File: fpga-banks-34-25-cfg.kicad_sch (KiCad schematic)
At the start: 49 parts, among them J13 PinHeader_1x3_P2.54mm_Drill1.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, Q12 2N7002_SOT-23-3, Q13 2N7002_SOT-23-3, Q14 2N7002_SOT-23-3, Q15 2N7002_SOT-23-3, Q16 2N7002_SOT-23-3, U14 XC7A100T-FGG484

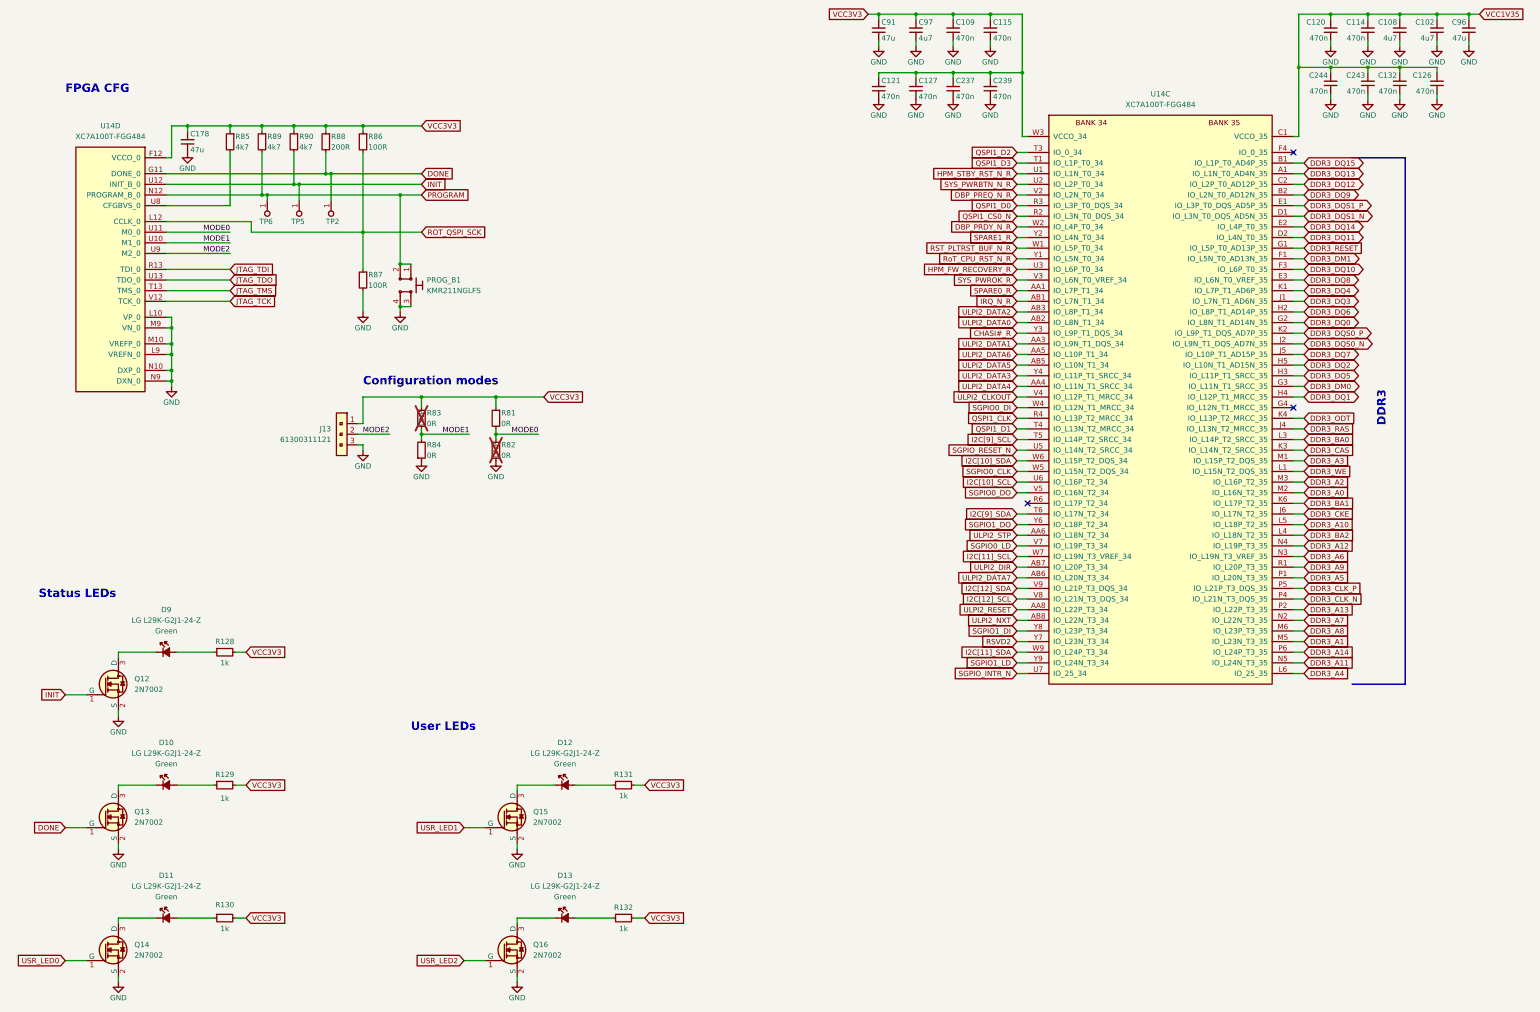
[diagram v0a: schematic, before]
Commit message: [#82378] Project refresh 81589
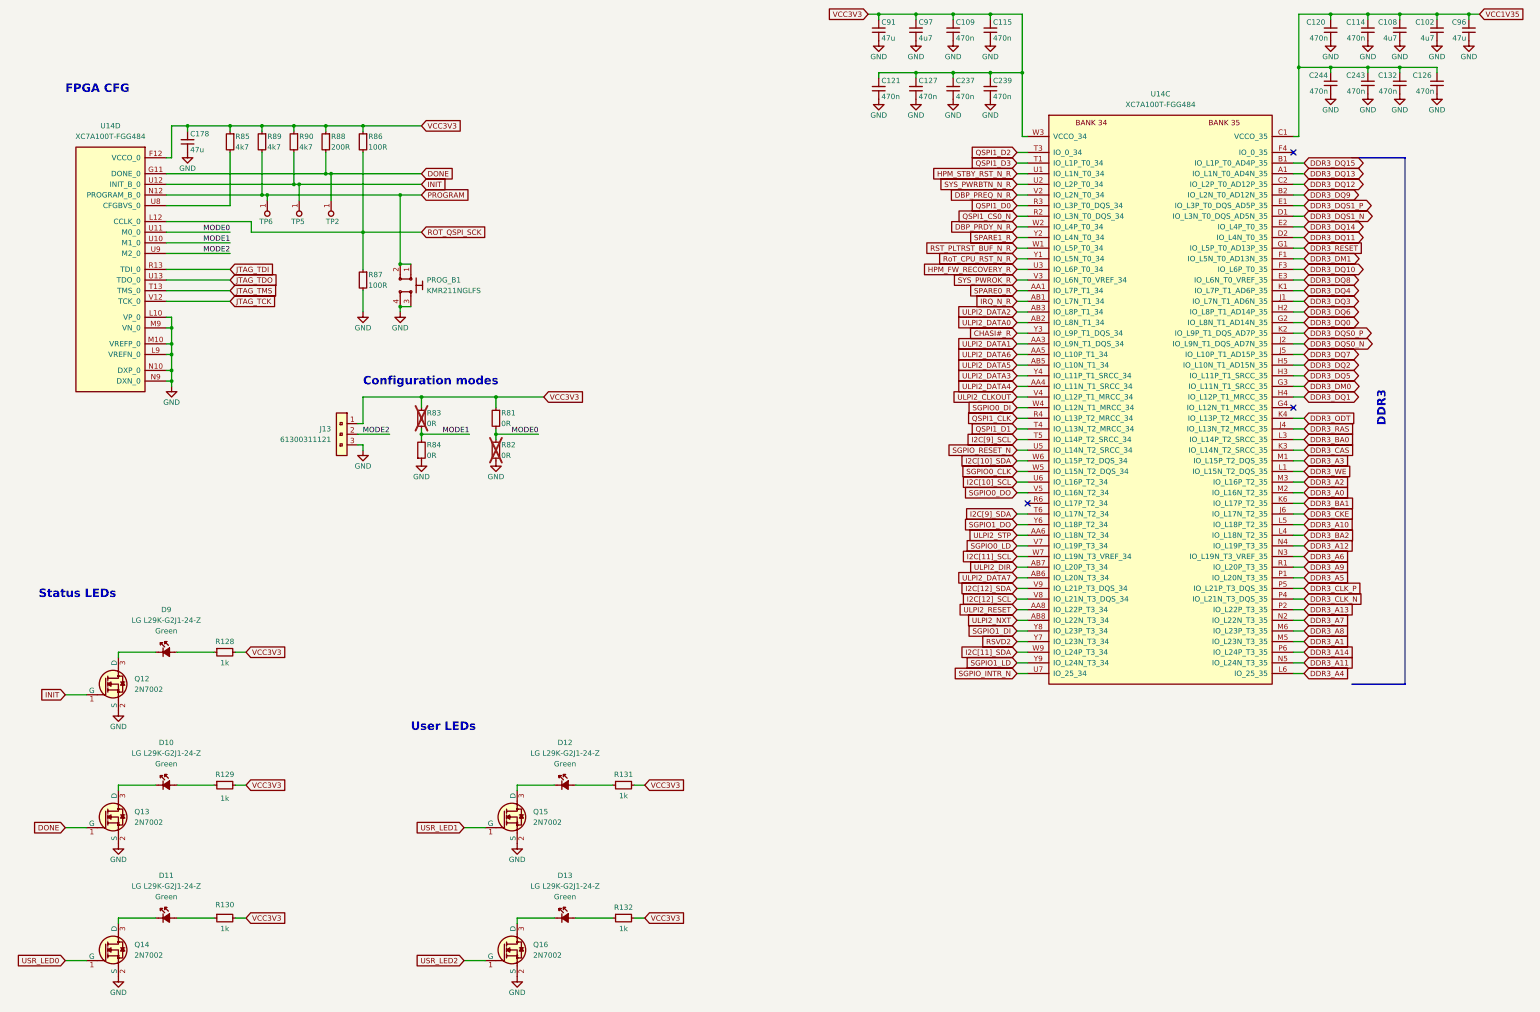
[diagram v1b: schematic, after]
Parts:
- R82, R83: DNP DNP -> (none)
